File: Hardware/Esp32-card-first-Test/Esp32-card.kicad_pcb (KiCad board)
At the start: 2 copper layers, 93 x 95 mm, 22 parts, among them J10 Conn_01x02_Pin, J11 Conn_01x02_Pin, J12 Conn_01x05_Pin, J13 Conn_01x02_Pin, J14 Conn_01x06_Pin, J2 Conn_01x02_Pin, J3 Conn_01x02_Pin, J4 Conn_01x03_Pin, J5 Conn_01x03_Pin, J6 Conn_01x02_Pin, J7 Conn_01x14_Socket, J8 Conn_01x06_Pin, J9 Conn_01x05_Pin, U1 74HC595, U2 74HC595, U4 74HC4051

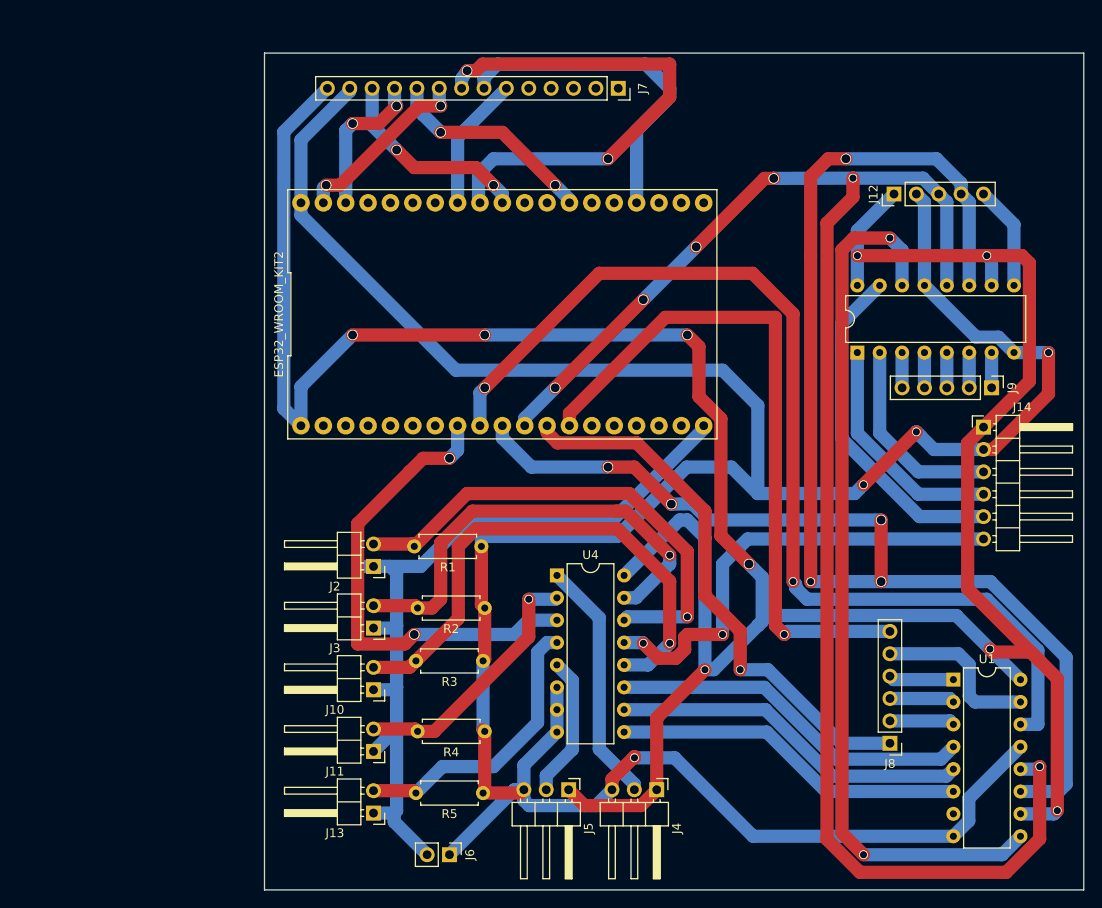
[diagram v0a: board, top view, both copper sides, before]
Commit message: pcb
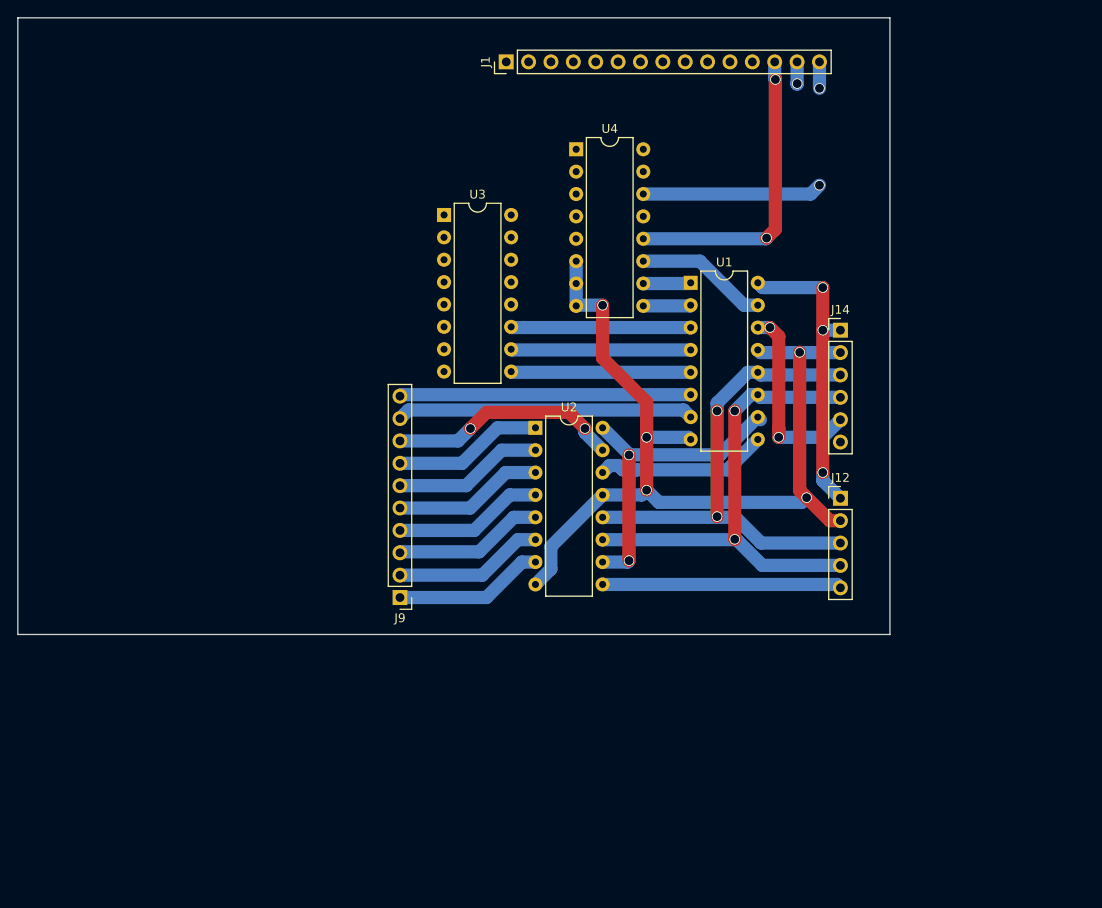
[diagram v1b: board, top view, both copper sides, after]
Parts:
- removed ESP32_WROOM_KIT2: ~, MyEsp32Library:Esp32_Wroom32_DevKit
- removed J10, J11, J13, J2, J3: Conn_01x02_Pin, Connector_PinHeader_2.54mm:PinHeader_1x02_P2.54mm_Horizontal
- removed J4, J5: Conn_01x03_Pin, Connector_PinHeader_2.54mm:PinHeader_1x03_P2.54mm_Horizontal
- removed J6: Conn_01x02_Pin, Connector_PinHeader_2.54mm:PinHeader_1x02_P2.54mm_Vertical
- removed J7: Conn_01x14_Socket, Connector_PinSocket_2.54mm:PinSocket_1x14_P2.54mm_Vertical
- removed J8: Conn_01x06_Pin, Connector_PinHeader_2.54mm:PinHeader_1x06_P2.54mm_Vertical
- removed R1, R2, R3, R4, R5: R, Resistor_THT:R_Axial_DIN0207_L6.3mm_D2.5mm_P7.62mm_Horizontal
- added J1: Conn_01x15_Pin, Connector_PinHeader_2.54mm:PinHeader_1x15_P2.54mm_Vertical, F.Cu at (143.4, 33.0)
- added U3: 74HC4051, Package_DIP:DIP-16_W7.62mm, F.Cu at (136.4, 50.4)
- J14: footprint Connector_PinHeader_2.54mm:PinHeader_1x06_P2.54mm_Horizontal -> Connector_PinHeader_2.54mm:PinHeader_1x06_P2.54mm_Vertical
- J9: value Conn_01x05_Pin -> Conn_01x10_Pin; footprint Connector_PinHeader_2.54mm:PinHeader_1x05_P2.54mm_Vertical -> Connector_PinHeader_2.54mm:PinHeader_1x10_P2.54mm_Vertical
- moved J9 71.3 mm to (131.4, 93.8), turned to 180 degrees
- moved U1 54.0 mm to (164.4, 58.1)
- moved U4 48.4 mm to (151.4, 42.9)
- moved U2 37.5 mm to (146.8, 74.5), turned to 0 degrees
- moved J12 35.1 mm to (181.4, 82.5), turned to 0 degrees
- moved J14 19.6 mm to (181.4, 63.5)
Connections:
- net GND renamed Net-(J12-Pin_2)
- J12 pad 3: Trig -> Net-(J12-Pin_3)
- J12 pad 4: Clock -> Net-(J12-Pin_4)
- J14 pad 3: Net-(J14-Pin_3) -> Net-(J12-Pin_3)
- J14 pad 4: Net-(J14-Pin_4) -> Net-(J12-Pin_4)
- U1 pad 1: M1_Pin_Dir2 -> Net-(U1-QB)
- U1 pad 11: Clock -> Net-(J12-Pin_4)
- U1 pad 12: Trig -> Net-(J12-Pin_3)
- U1 pad 14: Data -> Net-(J14-Pin_5)
- U1 pad 15: M1_Pin_Dir1 -> Net-(U1-QA)
- U1 pad 2: M2_Pin_Dir1 -> Net-(U1-QC)
- U1 pad 3: M2_Pin_Dir2 -> Net-(U1-QD)
- U1 pad 6: Net-(U1-QG) -> Net-(J9-Pin_10)
- U1 pad 7: unconnected-(U1-QH-Pad7) -> Net-(J9-Pin_9)
- U2 pad 1: Net-(J14-Pin_4) -> Net-(J9-Pin_7)
- U2 pad 11: Clock -> Net-(J12-Pin_4)
- U2 pad 12: Trig -> Net-(J12-Pin_3)
- U2 pad 15: Net-(J14-Pin_5) -> Net-(J9-Pin_8)
- U2 pad 2: Net-(J14-Pin_3) -> Net-(J9-Pin_6)
- U4 pad 1: Capteur_Hall_1 -> Net-(J1-Pin_12)
- U4 pad 10: Net-(U1-QF) -> Net-(U1-QB)
- U4 pad 11: Net-(U1-QE) -> Net-(U1-QA)
- U4 pad 12: Capteur_Force_3 -> Net-(J1-Pin_13)
- U4 pad 13: Net-(J14-Pin_6) -> Net-(U3-A)
- U4 pad 14: Capteur_Force_1 -> Net-(J1-Pin_15)
- U4 pad 15: Capteur_Force_2 -> Net-(J1-Pin_14)
- U4 pad 2: Capteur_Autre_1 -> Net-(J1-Pin_10)
- U4 pad 3: Analog_Pin1 -> Net-(J14-Pin_6)
- U4 pad 4: Capteur_Autre_2 -> Net-(J1-Pin_9)
- U4 pad 5: Capteur_Hall_2 -> Net-(J1-Pin_11)
- U4 pad 9: Net-(U1-QG) -> Net-(U1-QC)
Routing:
- net 3v3: track 340.0 -> 70.6 mm, vias 9 -> 5
- net Net-(J12-Pin_2): track 325.9 -> 105.0 mm, vias 4 -> 5
- net Trig: track 185.0 -> 0.00 mm, vias 6 -> 0
- net Clock: track 184.8 -> 0.00 mm, vias 6 -> 0
- net Data: track 118.9 -> 0.00 mm, vias 2 -> 0
- net 5v: track 93.5 -> 0.00 mm
- net Net-(U1-QH'): track 100.3 -> 19.6 mm, vias 2 -> 0
- net M1_Pin_EN: track 77.9 -> 0.00 mm, vias 1 -> 0
- net M2_Pin_EN: track 62.5 -> 0.00 mm, vias 1 -> 0
- net Capteur_Force_3: track 60.7 -> 0.00 mm, vias 1 -> 0
- net SCK: track 57.9 -> 0.00 mm, vias 2 -> 0
- net Net-(J12-Pin_3): track 0.00 -> 56.7 mm, vias 0 -> 2
- net Net-(J12-Pin_4): track 0.00 -> 55.7 mm, vias 0 -> 2
- net Capteur_Force_1: track 55.7 -> 0.00 mm, vias 1 -> 0
- net Analog_Pin1: track 55.0 -> 0.00 mm, vias 2 -> 0
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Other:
- board size 93 x 95 mm -> 99 x 70 mm
